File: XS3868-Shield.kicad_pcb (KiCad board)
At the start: 2 copper layers, 33 x 34.3 mm, 6 parts, among them P1 CONN_01X03, P2 CONN_01X02, U1 XS3868, U2 AP111733

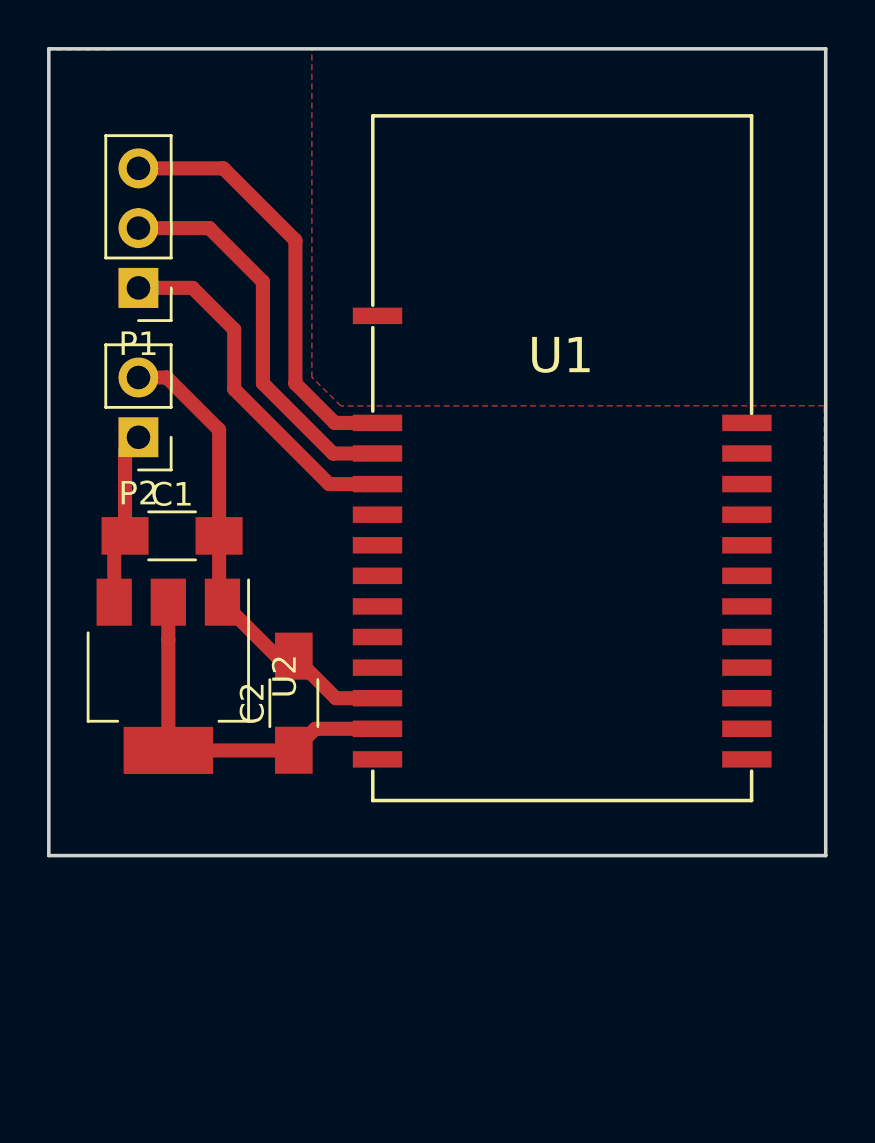
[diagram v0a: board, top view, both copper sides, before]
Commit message: Layout review
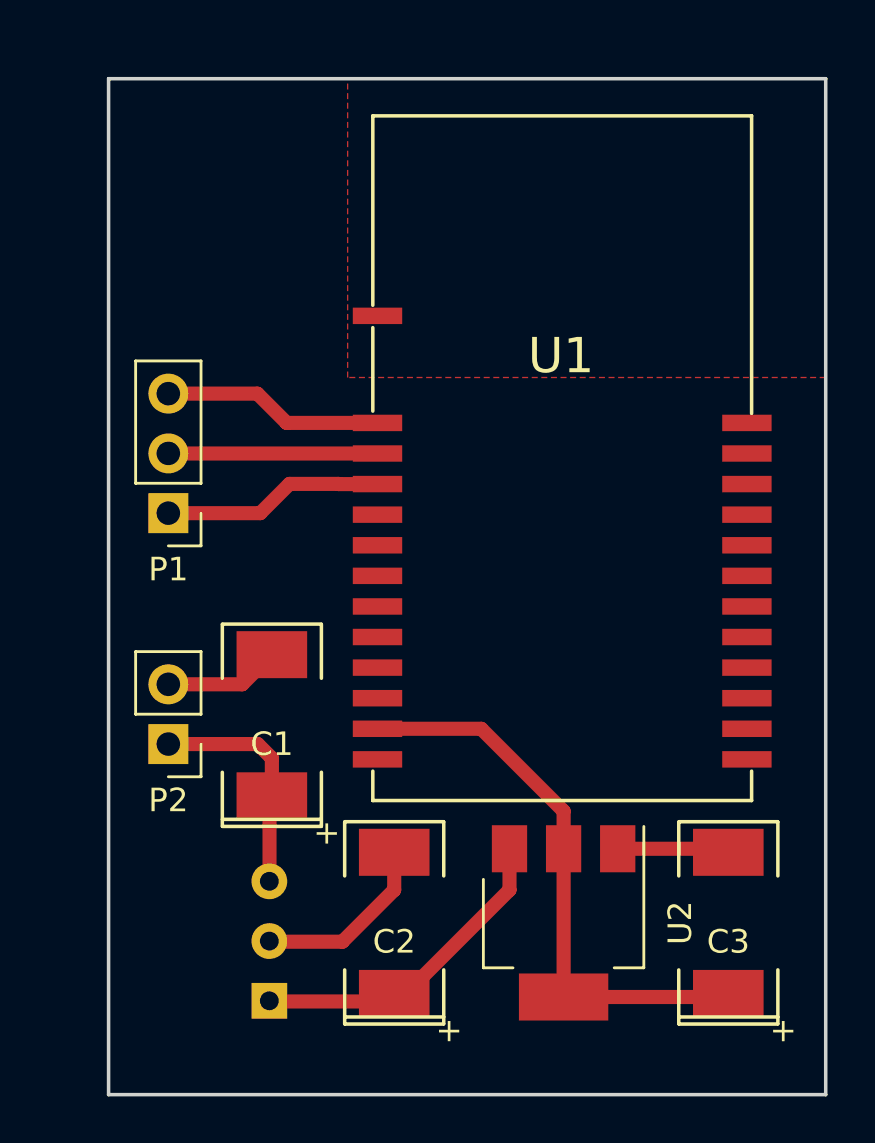
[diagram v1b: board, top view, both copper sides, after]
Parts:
- added C3: 100u, SMD_Packages:SMD-2512_Pol, F.Cu at (112.7, 68.9)
- added U3: LM7805, RACE_UP_ED:LM7805_TO92, B.Cu at (93.2, 72.2)
- C1, C2: footprint Capacitors_SMD:C_1206_HandSoldering -> SMD_Packages:SMD-2512_Pol
- moved U2 19.8 mm to (105.7, 68.9)
- moved P2 13.1 mm to (88.9, 61.3)
- moved C2 10.3 mm to (98.5, 68.9)
- moved P1 9.66 mm to (88.9, 51.5)
- moved C1 9.10 mm to (93.3, 60.5), turned to 90 degrees
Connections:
- C2 pad 1: +3V3 -> +5V
- U1 pad 1: Net-(U1-Pad1) -> (no net)
- U1 pad 10: Net-(U1-Pad10) -> (no net)
- U1 pad 13: Net-(U1-Pad13) -> (no net)
- U1 pad 14: Net-(U1-Pad14) -> (no net)
- U1 pad 15: Net-(U1-Pad15) -> (no net)
- U1 pad 16: Net-(U1-Pad16) -> (no net)
- U1 pad 17: Net-(U1-Pad17) -> (no net)
- U1 pad 18: Net-(U1-Pad18) -> (no net)
- U1 pad 19: Net-(U1-Pad19) -> (no net)
- U1 pad 20: Net-(U1-Pad20) -> (no net)
- U1 pad 21: Net-(U1-Pad21) -> (no net)
- U1 pad 22: Net-(U1-Pad22) -> (no net)
- U1 pad 23: Net-(U1-Pad23) -> (no net)
- U1 pad 24: Net-(U1-Pad24) -> (no net)
- U1 pad 25: Net-(U1-Pad25) -> (no net)
- U1 pad 5: Net-(U1-Pad5) -> (no net)
- U1 pad 6: Net-(U1-Pad6) -> (no net)
- U1 pad 7: Net-(U1-Pad7) -> (no net)
- U1 pad 8: Net-(U1-Pad8) -> (no net)
- U1 pad 9: Net-(U1-Pad9) -> (no net)
- U2 pad 3: +12V -> +5V
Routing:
- net +5V: track 0.00 -> 12.5 mm
- net Net-(P1-Pad3): track 18.2 -> 9.41 mm
- net +3V3: track 15.6 -> 24.3 mm
- net Net-(P1-Pad2): track 16.7 -> 8.89 mm
- net Net-(P1-Pad1): track 15.1 -> 9.41 mm
- net +12V: track 7.44 -> 11.3 mm
- net GND: track 20.0 -> 17.5 mm
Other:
- board size 33 x 34.3 mm -> 30.5 x 43.2 mm
